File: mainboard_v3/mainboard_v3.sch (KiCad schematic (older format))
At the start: 31 parts, among them J1 PWR_IN, J2 CLK_IN, J3 Conn_01x50, SW1 RESET, U1 DS1813, U2 W65C02SxP, U3 74HC21, U4 CY62256-70PC, U5 28C256, X1 ACO-xxxMHz

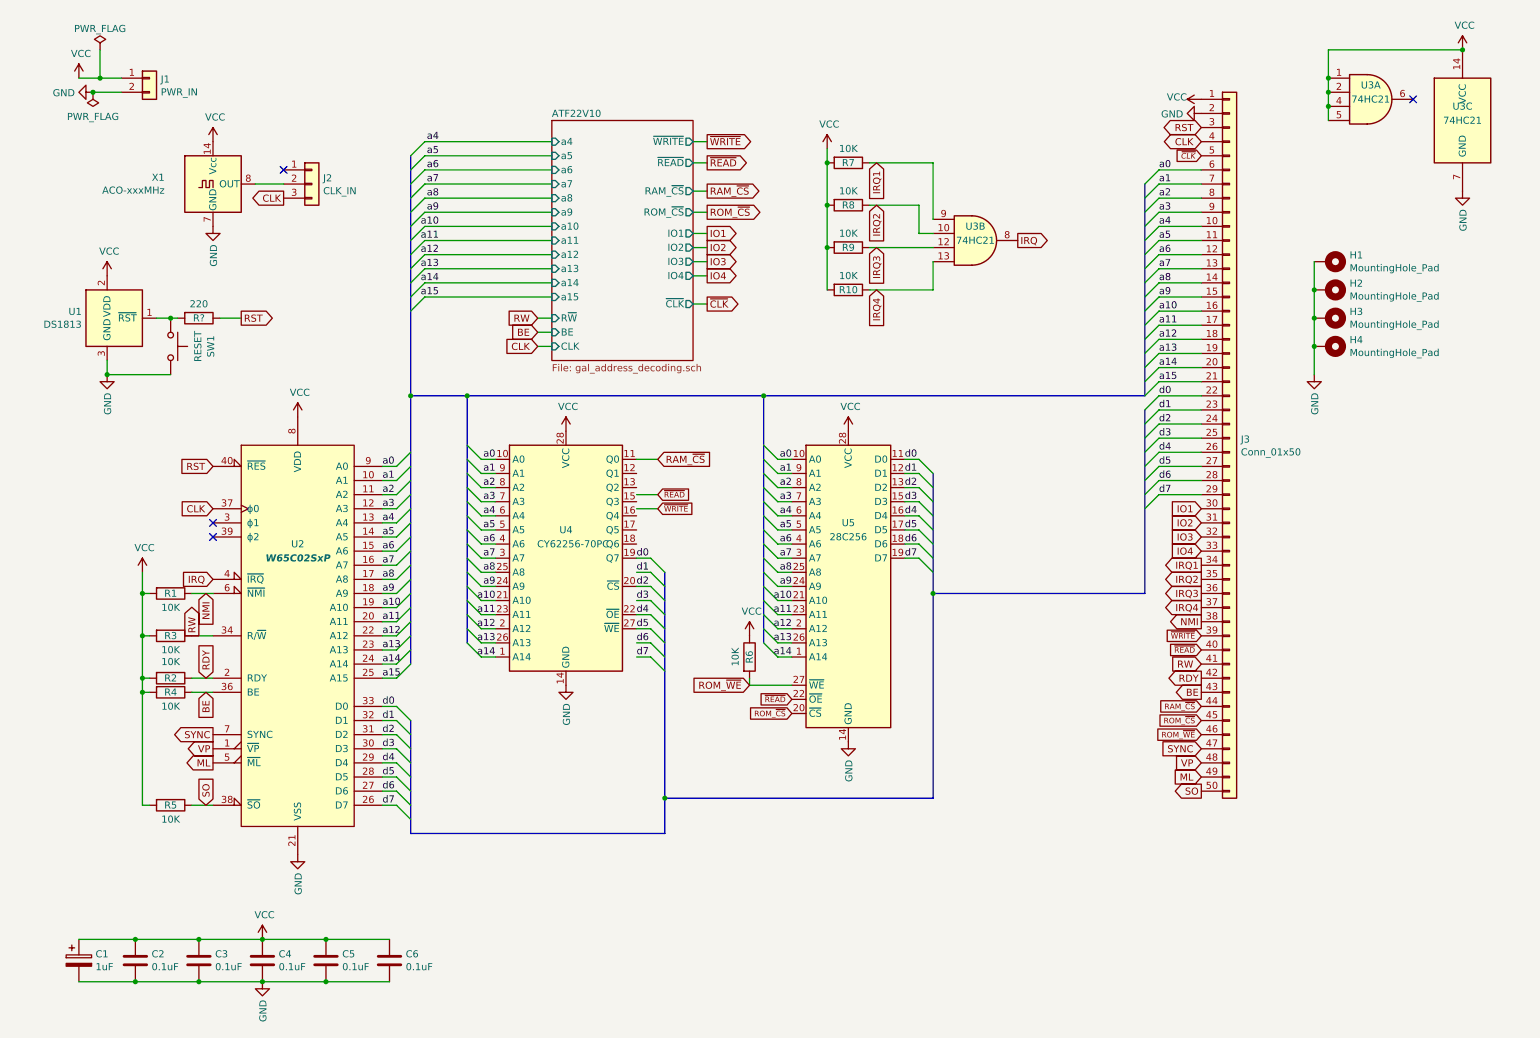
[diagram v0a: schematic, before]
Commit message: Mainboard v3
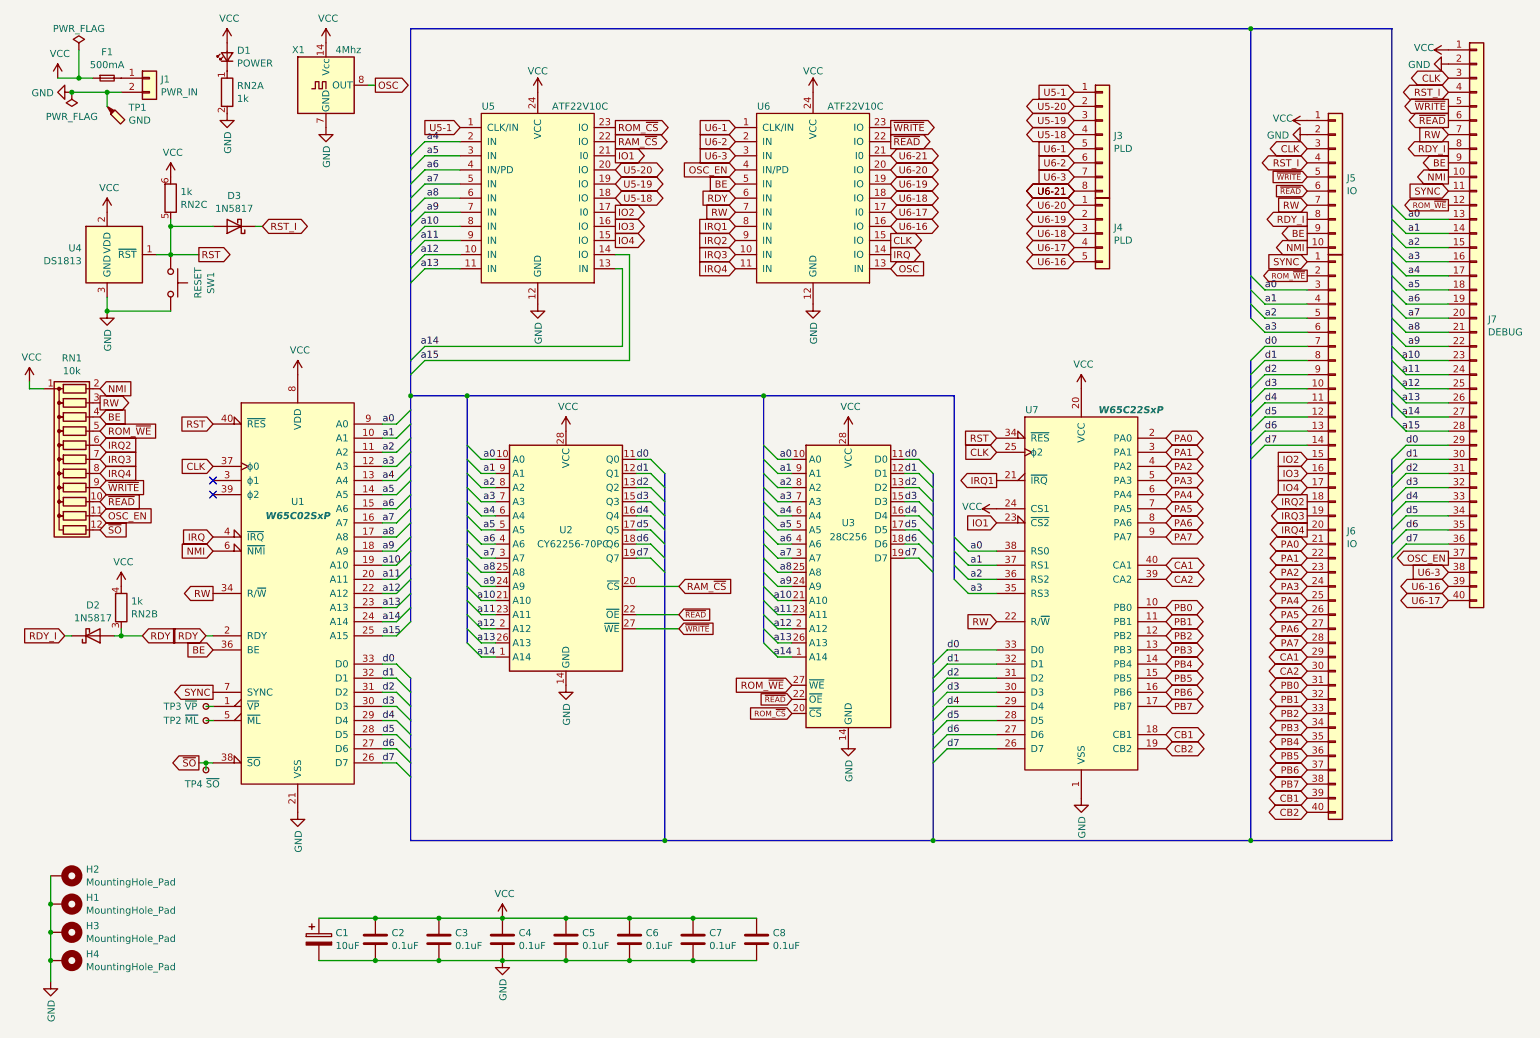
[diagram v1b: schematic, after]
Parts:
- removed J2: CLK_IN, Connector_PinSocket_2.54mm:PinSocket_1x03_P2.54mm_Vertical, symbol Connector_Generic:Conn_01x03
- removed J3: Conn_01x50, AK's_Footprints:PinSocket_1x50_P2.54mm_Vertical, symbol AK's_Library:Conn_01x50
- removed R1, R10, R2, R3, R4, R5, R6, R7, R8, R9: 10K, Resistor_THT:R_Axial_DIN0207_L6.3mm_D2.5mm_P7.62mm_Horizontal, symbol Device:R
- removed R?: 220, Resistor_THT:R_Axial_DIN0207_L6.3mm_D2.5mm_P7.62mm_Horizontal, symbol Device:R
- removed U3: 74HC21, Package_DIP:DIP-14_W7.62mm, symbol 74xx:74LS21
- added C7, C8: 0.1uF, Capacitor_THT:C_Disc_D3.0mm_W1.6mm_P2.50mm, symbol Device:C
- added D1: POWER, LED_THT:LED_D3.0mm, symbol Device:LED_Small
- added D2, D3: 1N5817, Diode_THT:D_DO-41_SOD81_P7.62mm_Horizontal, symbol Diode:1N5817
- added F1: 500mA, Fuse:Fuse_Littelfuse_372_D8.50mm, symbol Device:Fuse_Small
- added J3: PLD, Connector_PinSocket_2.54mm:PinSocket_1x08_P2.54mm_Vertical, symbol Connector_Generic:Conn_01x08
- added J4: PLD, Connector_PinSocket_2.54mm:PinSocket_1x05_P2.54mm_Vertical, symbol Connector_Generic:Conn_01x05
- added J5: IO, Connector_PinHeader_2.54mm:PinHeader_1x10_P2.54mm_Vertical, symbol Connector_Generic:Conn_01x10
- added J6: IO, Connector_PinHeader_2.54mm:PinHeader_1x40_P2.54mm_Vertical, symbol Connector_Generic:Conn_01x40
- added J7: DEBUG, Connector_IDC:IDC-Header_2x20_P2.54mm_Vertical, symbol Connector_Generic:Conn_01x40
- added RN1: 10k, Resistor_THT:R_Array_SIP12, symbol Device:R_Network11
- added RN2: 1k, Resistor_THT:R_Array_SIP6, symbol Device:R_Pack03_SIP_Split
- added TP1: GND, TestPoint:TestPoint_Loop_D2.60mm_Drill1.6mm_Beaded, symbol Connector:TestPoint_Probe
- added TP2: ~ML, TestPoint:TestPoint_THTPad_D1.5mm_Drill0.7mm, symbol Connector:TestPoint_Small
- added TP3: ~VP, TestPoint:TestPoint_THTPad_D1.5mm_Drill0.7mm, symbol Connector:TestPoint_Small
- added TP4: ~SO, TestPoint:TestPoint_THTPad_D1.5mm_Drill0.7mm, symbol Connector:TestPoint_Small
- added U5, U6: ATF22V10C, Socket:DIP_Socket-24_W4.3_W5.08_W7.62_W10.16_W10.9_3M_224-5248-00-0602J, symbol mainboard_v3:ATF22V10C
- added U7: W65C22SxP, Package_DIP:DIP-40_W15.24mm, symbol 65xx:W65C22SxP
- C1: value 1uF -> 10uF; footprint Capacitor_THT:CP_Radial_D4.0mm_P2.00mm -> Capacitor_THT:CP_Radial_D6.3mm_P2.50mm
- J1: footprint Connector_PinSocket_2.54mm:PinSocket_1x02_P2.54mm_Vertical -> Connector_JST:JST_EH_B2B-EH-A_1x02_P2.50mm_Vertical
- X1: value ACO-xxxMHz -> 4Mhz
- renumbered U2 to U1, U4 to U2, U5 to U3, U1 to U4
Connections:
- net BE: now also J5.9 (Pin_9), J7.9 (Pin_9), RN1.4 (R3), U6.5 (IN)
- net CLK: now also J5.3 (Pin_3), J7.3 (Pin_3), U6.15 (IO), U7.25 (ϕ2)
- net GND: now also C7.2, C8.2, J5.2 (Pin_2), J7.2 (Pin_2), RN2.2 (R1.2), TP1.1, U5.12 (GND), U6.12 (GND), U7.1 (VSS)
- net IO1: now also U5.21 (I0), U7.23 (~CS2)
- net IO2: now also J6.15 (Pin_15), U5.17 (I0)
- net IO3: now also J6.16 (Pin_16), U5.16 (IO)
- net IO4: now also J6.17 (Pin_17), U5.15 (IO)
- net IRQ: now also U6.14 (IO)
- net IRQ1: now also U6.8 (IN), U7.21 (~IRQ)
- net IRQ2: now also J6.18 (Pin_18), RN1.6 (R5), U6.9 (IN)
- net IRQ3: now also J6.19 (Pin_19), RN1.7 (R6), U6.10 (IN)
- net IRQ4: now also J6.20 (Pin_20), RN1.8 (R7), U6.11 (IN)
- net NMI: now also J5.10 (Pin_10), J7.10 (Pin_10), RN1.2 (R1)
- net RAM_~CS: now also U2.20 (~CS), U5.22 (IO); no longer U2.11 (Q0)
- net RDY: now also D2.2 (A), RN2.3 (R2.1), U6.6 (IN)
- net ROM_~CS: now also U5.23 (IO)
- net ROM_~WE: now also J6.2 (Pin_2), J7.12 (Pin_12), RN1.5 (R4)
- net RST: now also SW1.1, U4.1 (~RST), D3.2 (A), RN2.5 (R3.1), U7.34 (~RES)
- net RW: now also J5.7 (Pin_7), J7.7 (Pin_7), RN1.3 (R2), U6.7 (IN), U7.22 (R/~W)
- net SYNC: now also J6.1 (Pin_1), J7.11 (Pin_11)
- net VCC: now also C7.1, C8.1, D1.2 (A), F1.1, J5.1 (Pin_1), J7.1 (Pin_1), RN1.1 (common), RN2.4 (R2.2), RN2.6 (R3.2), U5.24 (VCC), U6.24 (VCC), U7.20 (VCC), U7.24 (CS1); no longer J1.1 (Pin_1)
- net a0: now also J6.3 (Pin_3), J7.13 (Pin_13), U7.38 (RS0)
- net a1: now also J6.4 (Pin_4), J7.14 (Pin_14), U7.37 (RS1)
- net a10: now also J7.23 (Pin_23), U5.8 (IN)
- net a11: now also J7.24 (Pin_24), U5.9 (IN)
- net a12: now also J7.25 (Pin_25), U5.10 (IN)
- net a13: now also J7.26 (Pin_26), U5.11 (IN)
- net a14: now also J7.27 (Pin_27), U5.13 (IN)
- net a15: now also J7.28 (Pin_28), U5.14 (IO)
- net a2: now also J6.5 (Pin_5), J7.15 (Pin_15), U7.36 (RS2)
- net a3: now also J6.6 (Pin_6), J7.16 (Pin_16), U7.35 (RS3)
- net a4: now also J7.17 (Pin_17), U5.2 (IN)
- net a5: now also J7.18 (Pin_18), U5.3 (IN)
- net a6: now also J7.19 (Pin_19), U5.4 (IN/PD)
- net a7: now also J7.20 (Pin_20), U5.5 (IN)
- net a8: now also J7.21 (Pin_21), U5.6 (IN)
- net a9: now also J7.22 (Pin_22), U5.7 (IN)
- net d0: now also U2.11 (Q0), J6.7 (Pin_7), J7.29 (Pin_29), U7.33 (D0); no longer U2.19 (Q7)
- net d1: now also U2.12 (Q1), J6.8 (Pin_8), J7.30 (Pin_30), U7.32 (D1)
- net d2: now also U2.13 (Q2), J6.9 (Pin_9), J7.31 (Pin_31), U7.31 (D2); no longer U2.20 (~CS)
- net d3: now also U2.15 (Q3), J6.10 (Pin_10), J7.32 (Pin_32), U7.30 (D3)
- net d4: now also U2.16 (Q4), J6.11 (Pin_11), J7.33 (Pin_33), U7.29 (D4); no longer U2.22 (~OE)
- net d5: now also U2.17 (Q5), J6.12 (Pin_12), J7.34 (Pin_34), U7.28 (D5); no longer U2.27 (~WE)
- net d6: now also U2.18 (Q6), J6.13 (Pin_13), J7.35 (Pin_35), U7.27 (D6)
- net d7: now also U2.19 (Q7), J6.14 (Pin_14), J7.36 (Pin_36), U7.26 (D7)
- net ~READ: now also U2.22 (~OE), J5.6 (Pin_6), J7.6 (Pin_6), RN1.10 (R9), U6.22 (IO)
- net ~WRITE: now also U2.27 (~WE), J5.5 (Pin_5), J7.5 (Pin_5), RN1.9 (R8), U6.23 (IO)
- net OSC: now reaches X1.8 (OUT)
- net OSC: now also U6.13 (IN)
- net ML: no longer names the net of U1.5 (~ML)
- net ML: now also TP2.1
- net SO renamed ~SO
- net ~SO: now also RN1.12 (R11), TP4.1
- net VP: no longer names the net of U1.1 (~VP)
- net VP: now also TP3.1
- new net: D1.1 (K), RN2.1 (R1.1)
- new net: F1.2, J1.1 (Pin_1)
- new net CA1: J6.29 (Pin_29), U7.40 (CA1)
- new net CA2: J6.30 (Pin_30), U7.39 (CA2)
- new net CB1: J6.39 (Pin_39), U7.18 (CB1)
- new net CB2: J6.40 (Pin_40), U7.19 (CB2)
- new net OSC_EN: J7.37 (Pin_37), RN1.11 (R10), U6.4 (IN/PD)
- new net PA0: J6.21 (Pin_21), U7.2 (PA0)
- new net PA1: J6.22 (Pin_22), U7.3 (PA1)
- new net PA2: J6.23 (Pin_23), U7.4 (PA2)
- new net PA3: J6.24 (Pin_24), U7.5 (PA3)
- new net PA4: J6.25 (Pin_25), U7.6 (PA4)
- new net PA5: J6.26 (Pin_26), U7.7 (PA5)
- new net PA6: J6.27 (Pin_27), U7.8 (PA6)
- new net PA7: J6.28 (Pin_28), U7.9 (PA7)
- new net PB0: J6.31 (Pin_31), U7.10 (PB0)
- new net PB1: J6.32 (Pin_32), U7.11 (PB1)
- new net PB2: J6.33 (Pin_33), U7.12 (PB2)
- new net PB3: J6.34 (Pin_34), U7.13 (PB3)
- new net PB4: J6.35 (Pin_35), U7.14 (PB4)
- new net PB5: J6.36 (Pin_36), U7.15 (PB5)
- new net PB6: J6.37 (Pin_37), U7.16 (PB6)
- new net PB7: J6.38 (Pin_38), U7.17 (PB7)
- new net RDY_I: D2.1 (K), J5.8 (Pin_8), J7.8 (Pin_8)
- new net RST_I: D3.1 (K), J5.4 (Pin_4), J7.4 (Pin_4)
- new net U5-1: J3.1 (Pin_1), U5.1 (CLK/IN)
- new net U5-18: J3.4 (Pin_4), U5.18 (IO)
- new net U5-19: J3.3 (Pin_3), U5.19 (IO)
- new net U5-20: J3.2 (Pin_2), U5.20 (IO)
- new net U6-1: J3.5 (Pin_5), U6.1 (CLK/IN)
- new net U6-16: J4.5 (Pin_5), J7.39 (Pin_39), U6.16 (IO)
- new net U6-17: J4.4 (Pin_4), J7.40 (Pin_40), U6.17 (I0)
- new net U6-18: J4.3 (Pin_3), U6.18 (IO)
- new net U6-19: J4.2 (Pin_2), U6.19 (IO)
- new net U6-2: J3.6 (Pin_6), U6.2 (IN)
- new net U6-20: J4.1 (Pin_1), U6.20 (IO)
- new net U6-21: J3.8 (Pin_8), U6.21 (I0)
- new net U6-3: J3.7 (Pin_7), J7.38 (Pin_38), U6.3 (IN)
- no-connect marks 4 -> 2
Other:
- moved on the sheet: C1, C2, C3, C4, C5, C6, H1, H2, H3, H4, SW1, U1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
